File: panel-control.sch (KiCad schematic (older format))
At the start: 60 parts, among them J1 POWER_CONN, J2 SWIM, J3 PWR, J4 40HAT, J5 HUB-75_A, J6 HUB-75_B, J7 VBAT, J8 FAN, J9 MK_R, Q1 DMMT5401, Q2 DMG2305UX, Q3 AO4407A, Q4 S8050, SW1 POW, SW2 NRST, U1 TXS0108EPW, U2 TXS0108EPW, U3 TXS0108EPW, U4 HT7533-1, U5 STM8S103F3P

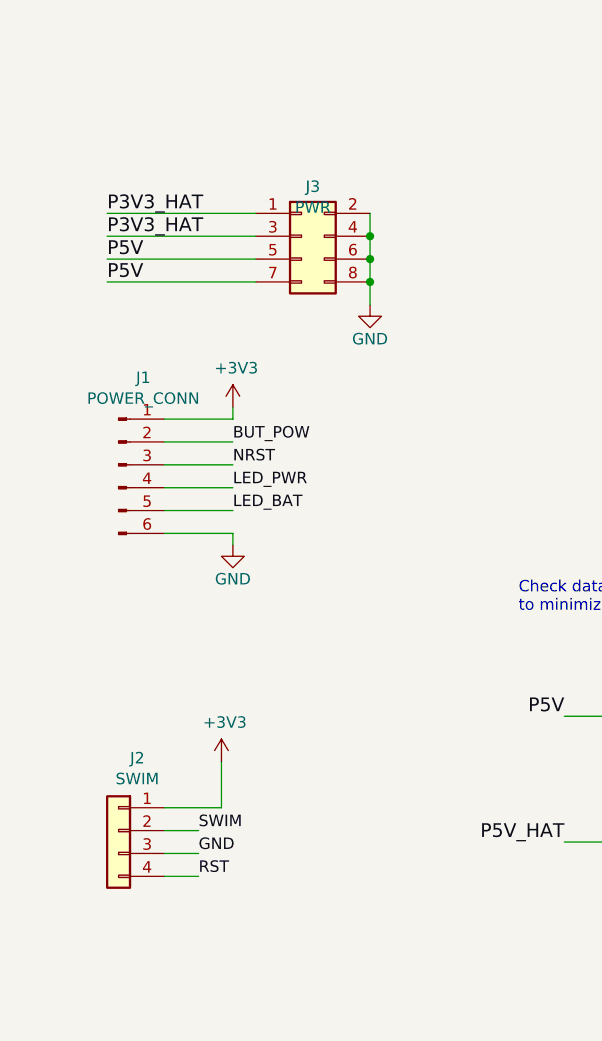
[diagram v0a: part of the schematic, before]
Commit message: sort of finished layout
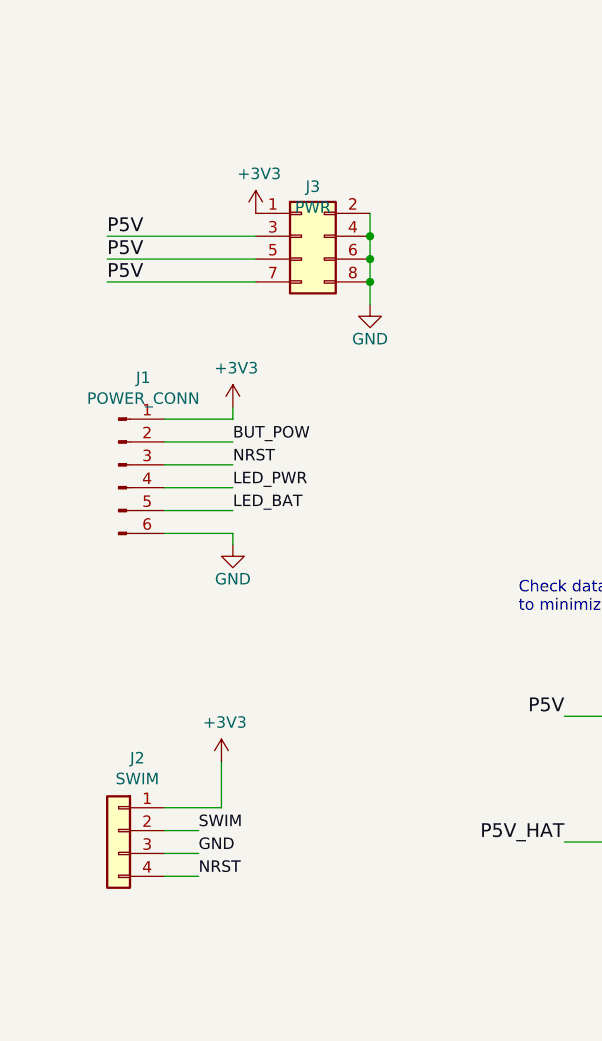
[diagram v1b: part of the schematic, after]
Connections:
- net RST is gone; now on net NRST: J2.4 (Pin_4)
- net +3.3VA: no longer J3.1 (Pin_1), J3.3 (Pin_3)
- net +3V3: now also J3.1 (Pin_1)
- net +5VA: now also J3.3 (Pin_3)
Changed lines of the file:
@@
 Text Label 1100 7150 0    60   ~ 0
 P5V
-Text Label 1100 7050 0    60   ~ 0
-P3V3_HAT
 Wire Wire Line
 	1100 7050 1750 7050
@@
 Wire Wire Line
 	4950 6600 5350 6600
-Text Label 1100 6950 0    60   ~ 0
-P3V3_HAT
 Text Label 1100 7250 0    60   ~ 0
 P5V
@@
 Wire Wire Line
 	2250 7250 2250 7350
-Wire Wire Line
-	1100 6950 1750 6950
 Wire Wire Line
 	1100 7250 1750 7250
@@
 	1350 9750 1500 9750
 Text Label 1500 9850 0    50   ~ 0
-RST
+NRST
 Wire Wire Line
 	1350 9850 1500 9850
@@
 Text Label 4000 6600 0    50   ~ 0
 R1B_B
+Text Label 1100 7050 0    60   ~ 0
+P5V
+$Comp
+L power:+3V3 #PWR0101
+U 1 1 5FFA1320
+P 1750 6950
+F 0 "#PWR0101" H 1750 6800 50  0001 C CNN
+F 1 "+3V3" H 1765 7123 50  0000 C CNN
+F 2 "" H 1750 6950 50  0001 C CNN
+F 3 "" H 1750 6950 50  0001 C CNN
+	1    1750 6950
+	1    0    0    -1
+$EndComp
 $EndSCHEMATC
